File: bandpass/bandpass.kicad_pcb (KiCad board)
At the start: 2 copper layers, 100 x 100 mm, 24 parts, among them J1 RX, J3 Conn_Coaxial, K2 G6K-2, K3 G6K-2, K4 G6K-2, K5 G6K-2, K6 G6K-2, K7 G6K-2, K8 G6K-2, P1 PMOD-Device-x2-Type-Generic-A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, X1 40 m, X2 15 m, X3 30 m, X4 12 m, X5 20 m, X6 10 m, X7 17 m

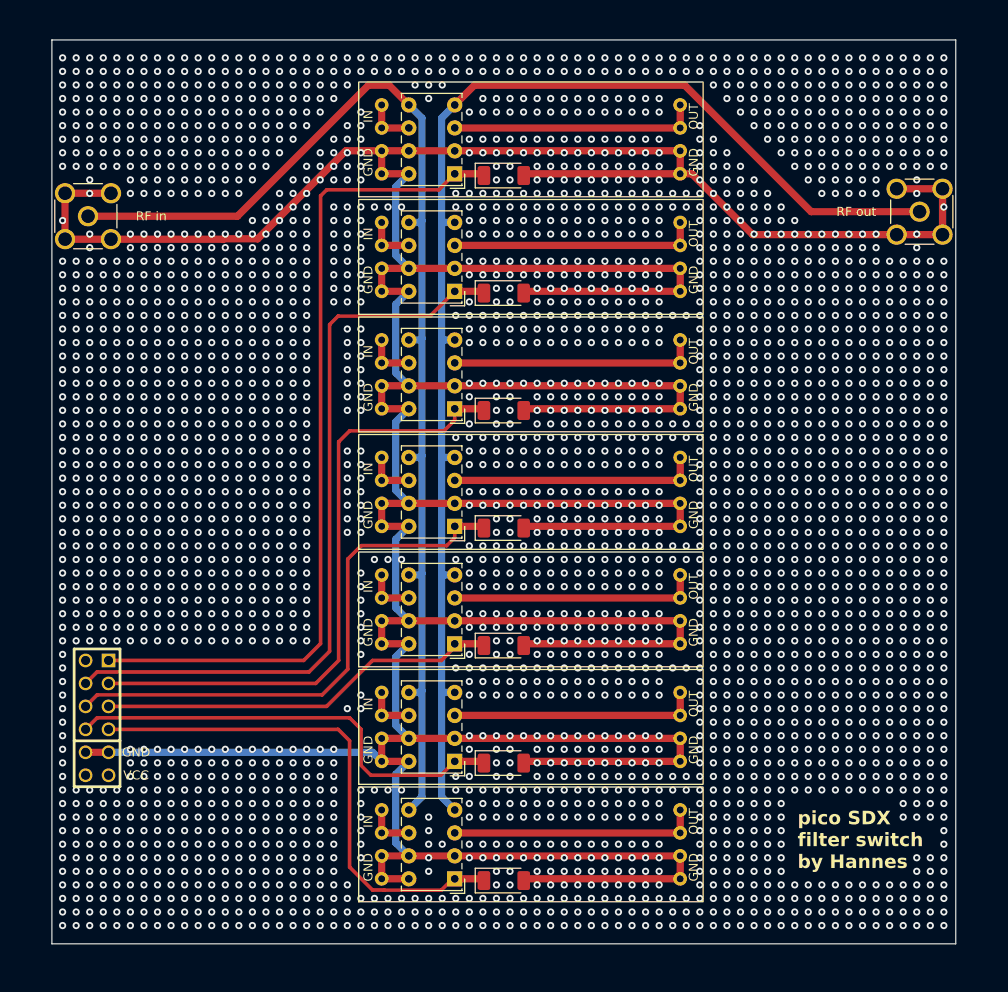
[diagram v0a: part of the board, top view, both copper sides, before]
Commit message: drc clean
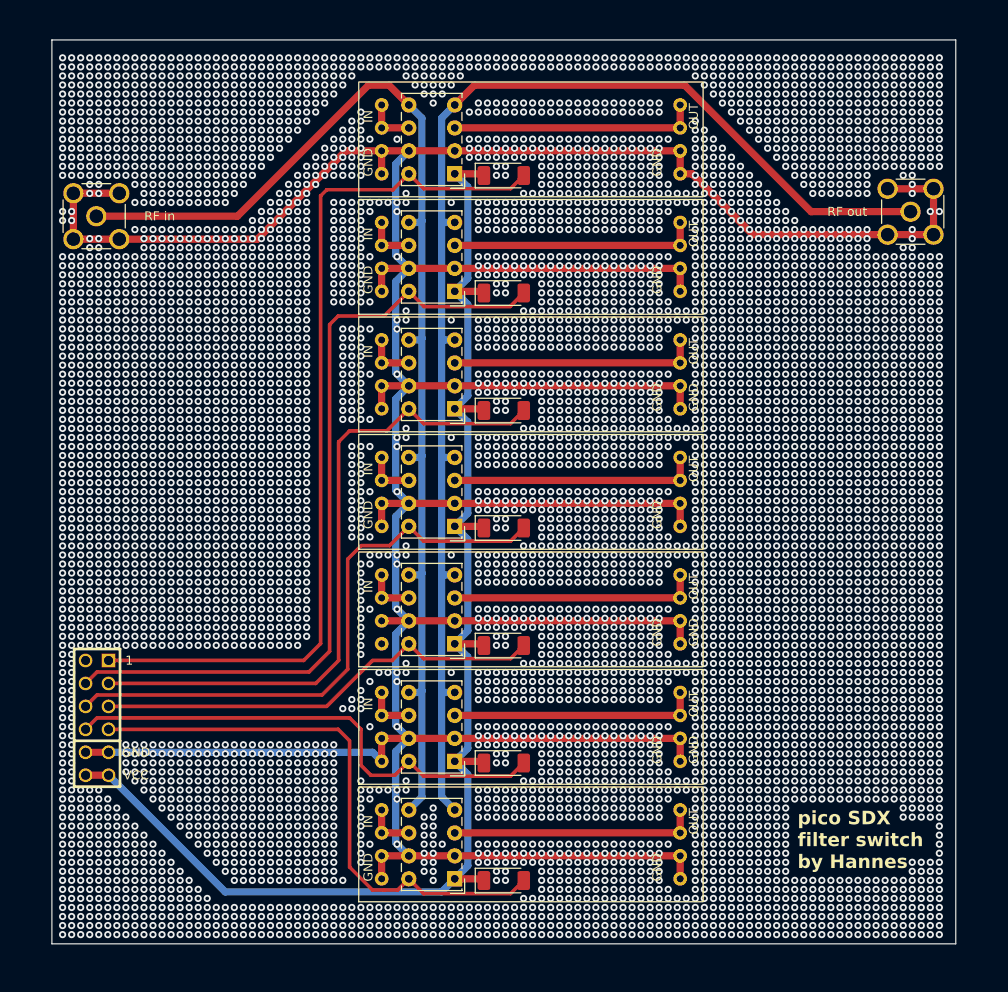
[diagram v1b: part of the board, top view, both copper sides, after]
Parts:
- moved J1 1.00 mm to (110.7, 36.2)
- moved J3 0.92 mm to (20.7, 36.7)
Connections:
- D2 pad 1: 40 m -> +12V
- D2 pad 2: GND -> 40 m
- D3 pad 1: 15 m -> +12V
- D3 pad 2: GND -> 15 m
- D4 pad 1: 30 m -> +12V
- D4 pad 2: GND -> 30 m
- D5 pad 1: 12 m -> +12V
- D5 pad 2: GND -> 12 m
- D6 pad 1: 20 m -> +12V
- D6 pad 2: GND -> 20 m
- D7 pad 1: 10 m -> +12V
- D7 pad 2: GND -> 10 m
- D8 pad 1: 17 m -> +12V
- D8 pad 2: GND -> 17 m
- K2 pad 1: 40 m -> +12V
- K2 pad 8: GND -> 40 m
- K3 pad 1: 15 m -> +12V
- K3 pad 8: GND -> 15 m
- K4 pad 1: 30 m -> +12V
- K4 pad 8: GND -> 30 m
- K5 pad 1: 12 m -> +12V
- K5 pad 8: GND -> 12 m
- K6 pad 1: 20 m -> +12V
- K6 pad 8: GND -> 20 m
- K7 pad 1: 10 m -> +12V
- K7 pad 8: GND -> 10 m
- K8 pad 1: 17 m -> +12V
- K8 pad 8: GND -> 17 m
- P1 pad 12: unconnected-(P1-P12-Pad12) -> +12V
- P1 pad 6: unconnected-(P1-P6-Pad6) -> +12V
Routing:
- net +12V: track 0.00 -> 155.8 mm
- net GND: track 603.8 -> 473.8 mm, vias 3170 -> 6833
- net 12 m: track 83.3 -> 89.2 mm
- net 10 m: track 92.9 -> 98.8 mm
- net 30 m: track 50.3 -> 56.2 mm
- net 40 m: track 57.7 -> 63.5 mm
- net 20 m: track 44.7 -> 50.3 mm
- net 17 m: track 60.3 -> 65.4 mm
- net 15 m: track 69.1 -> 74.2 mm
- net /Bandpass Filter/RF in: track 145.0 -> 144.0 mm
- net /Bandpass Filter/RF out: track 129.2 -> 128.3 mm
